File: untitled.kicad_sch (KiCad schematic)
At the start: 76 parts, among them U11 STP16CPC26T

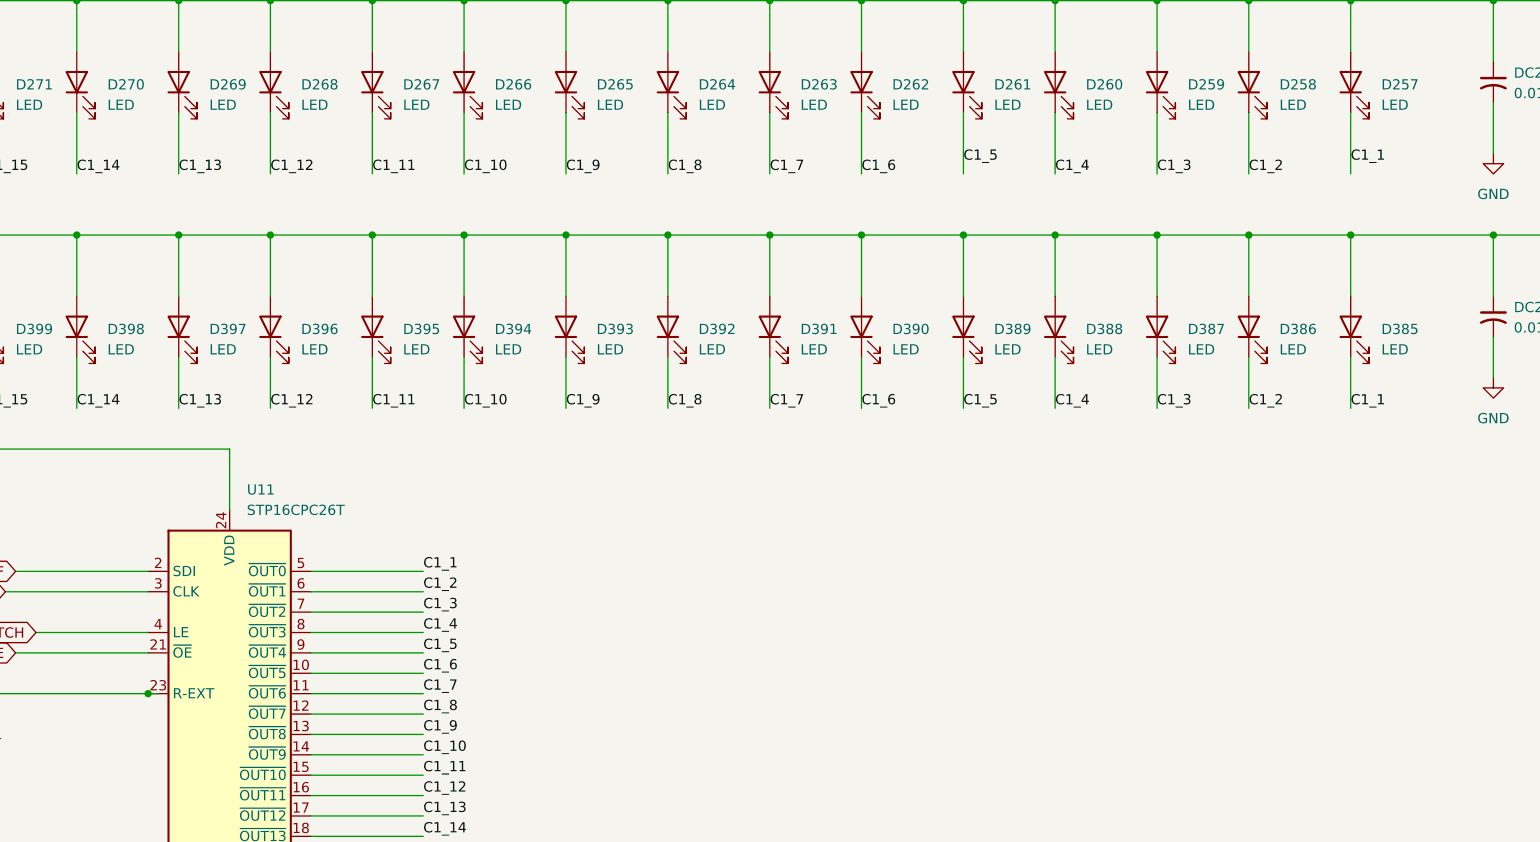
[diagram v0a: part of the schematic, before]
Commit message: sample
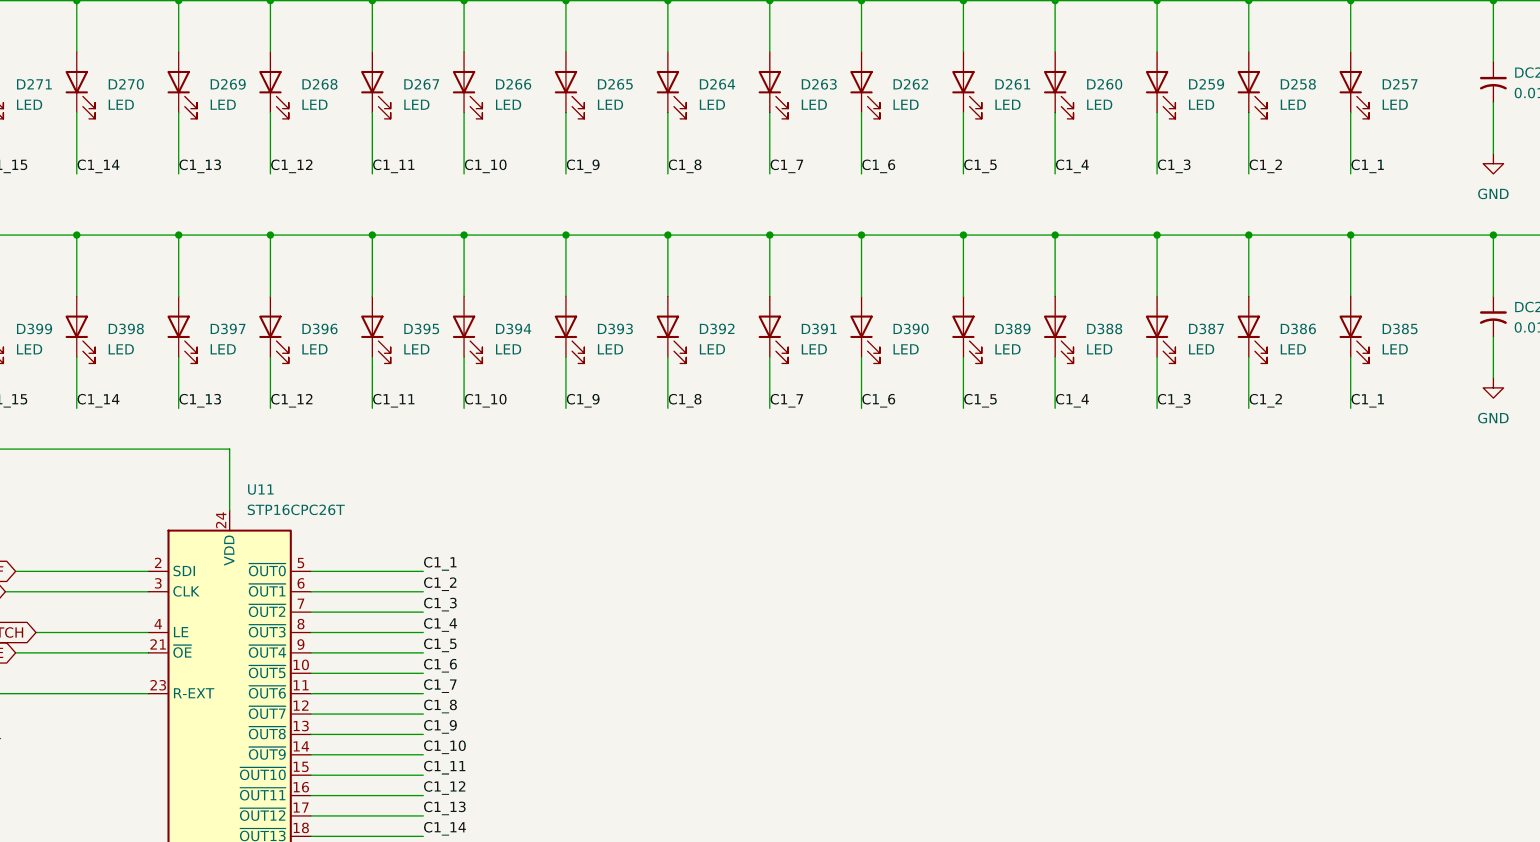
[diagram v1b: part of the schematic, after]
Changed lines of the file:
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@@
 	)
 	(junction
-		(at 82.55 158.75)
-		(diameter 0)
-		(color 0 0 0 0)
-	)
-	(junction
 		(at 73.66 72.39)
 		(diameter 0)
@@
 	(wire
 		(pts
-			(xy 58.42 158.75) (xy 82.55 158.75)
-		)
-		(stroke
-			(width 0)
-			(type default)
-		)
-	)
-	(wire
-		(pts
 			(xy 232.41 46.99) (xy 232.41 50.8)
 		)
@@
 	(wire
 		(pts
-			(xy 184.15 86.36) (xy 184.15 93.98)
-		)
-		(stroke
-			(width 0)
-			(type default)
-		)
-	)
-	(wire
-		(pts
 			(xy 232.41 86.36) (xy 232.41 93.98)
 		)
@@
 	(wire
 		(pts
+			(xy 184.15 86.36) (xy 184.15 93.98)
+		)
+		(stroke
+			(width 0)
+			(type default)
+		)
+	)
+	(wire
+		(pts
 			(xy 134.62 31.75) (xy 134.62 39.37)
 		)
@@
 	(wire
 		(pts
-			(xy 82.55 158.75) (xy 83.82 158.75)
-		)
-		(stroke
-			(width 0)
-			(type default)
-		)
-	)
-	(wire
-		(pts
 			(xy 26.67 115.57) (xy 26.67 120.65)
 		)
@@
 	(wire
 		(pts
+			(xy 58.42 158.75) (xy 82.55 158.75)
+		)
+		(stroke
+			(width 0)
+			(type default)
+		)
+	)
+	(wire
+		(pts
 			(xy 184.15 101.6) (xy 184.15 109.22)
 		)
@@
 	)
 	(label "C1_5"
-		(at 184.15 92.71 0)
+		(at 184.15 93.98 0)
 		(effects
 			(font
@@
 	)
 	(label "C1_1"
-		(at 232.41 92.71 0)
+		(at 232.41 93.98 0)
 		(effects
 			(font
